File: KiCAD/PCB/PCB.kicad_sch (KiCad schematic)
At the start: 20 parts, among them J1 XLR3_AudioJack3_Combo_Switch, J2 Conn_01x04, J3 Conn_01x04, SW1 RotaryEncoder_Switch, U1 ESP32-WROOM-32D, U2 MPU-6050, U3 MIC5219-3.3YM5

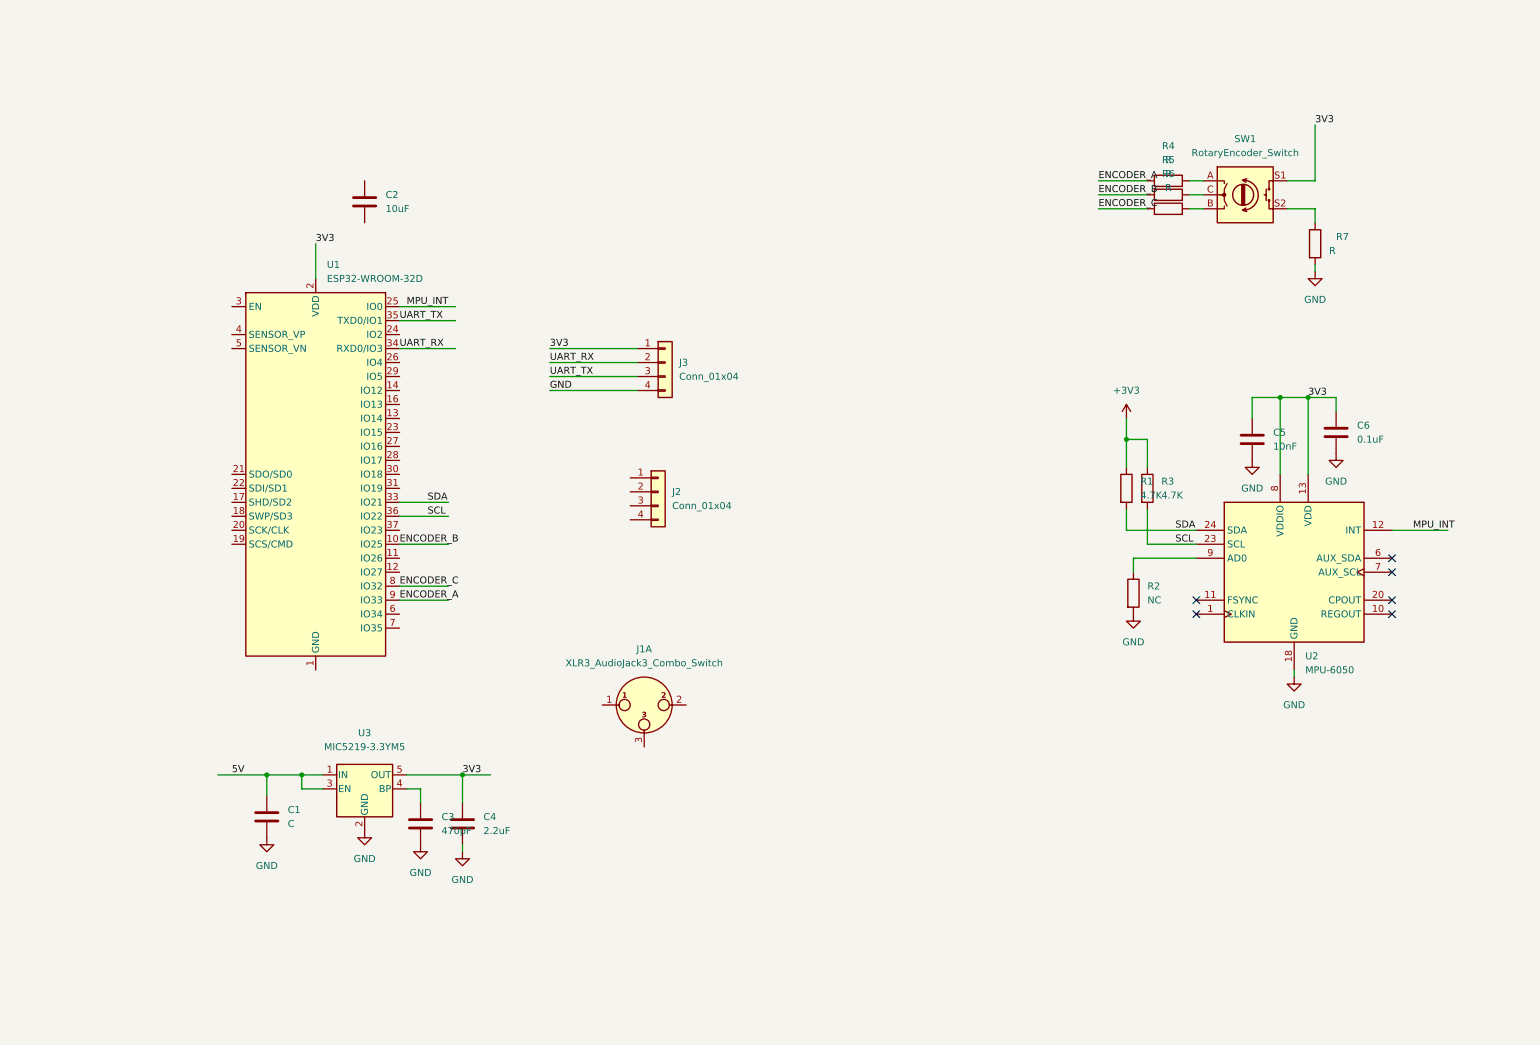
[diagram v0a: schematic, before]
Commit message: 原理圖第一版完成
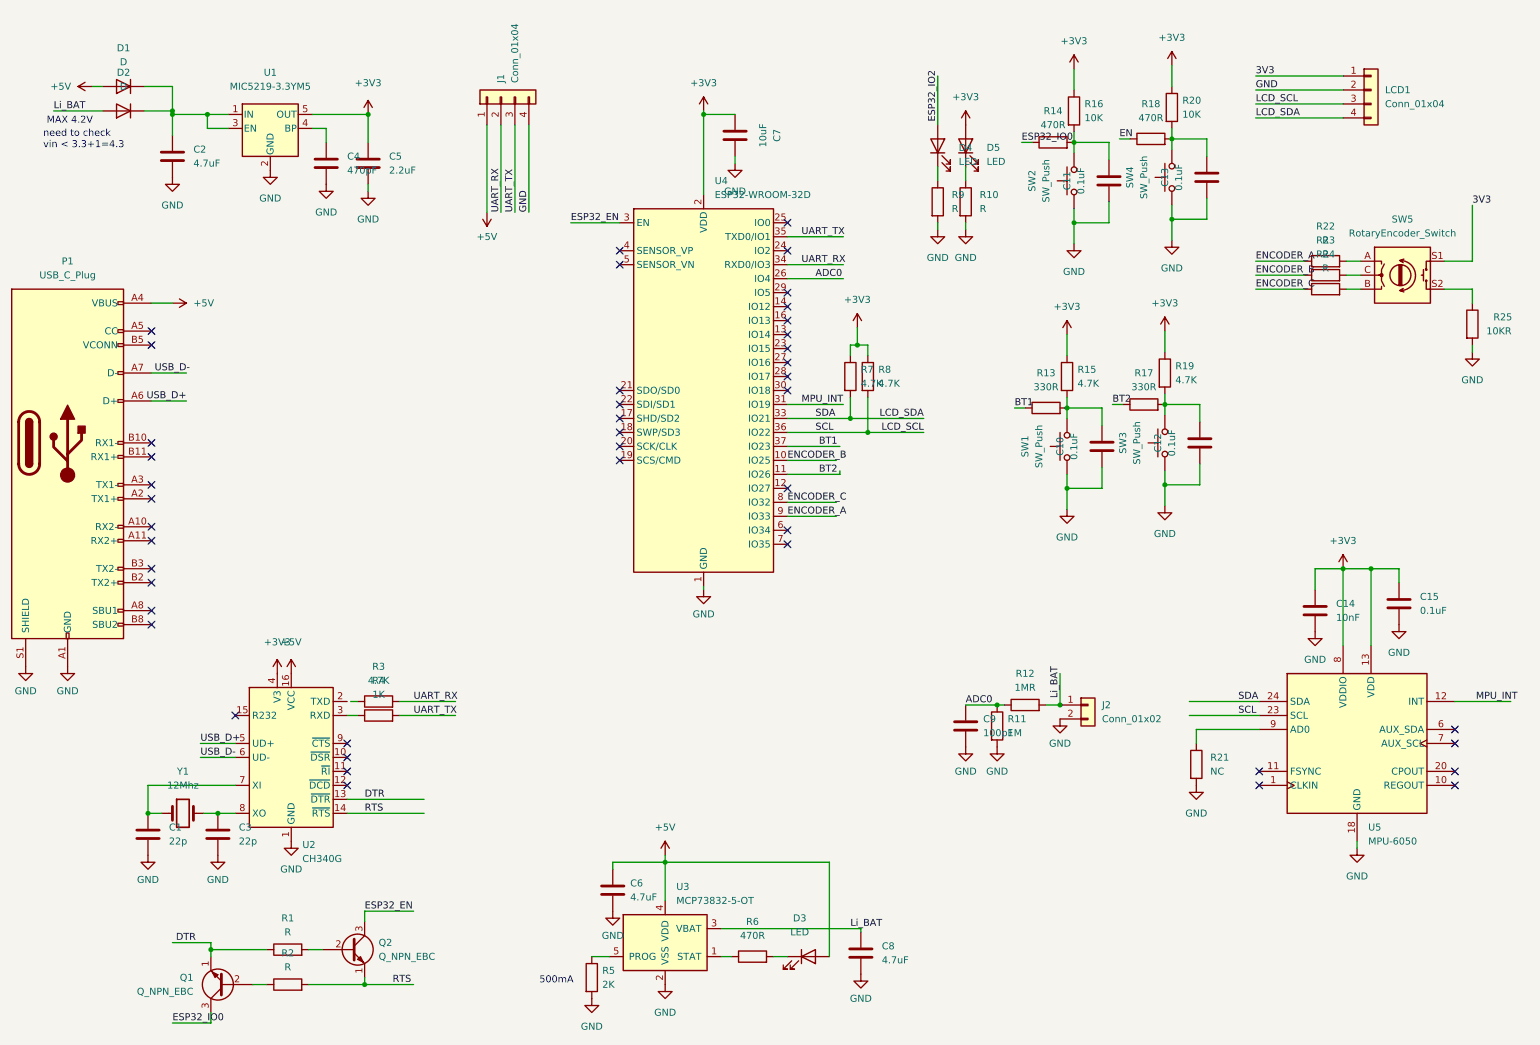
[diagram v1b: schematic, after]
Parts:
- removed J1: XLR3_AudioJack3_Combo_Switch, Button_Switch_THT:SW_E-Switch_EG2219_DPDT_Angled, symbol Connector:XLR3_AudioJack3_Combo_Switch
- added C1, C3: 22p, Capacitor_SMD:C_0603_1608Metric, symbol Device:C
- added C10, C11, C12, C13: 0.1uF, Capacitor_SMD:C_0603_1608Metric, symbol Device:C
- added C6, C8: 4.7uF, Capacitor_SMD:C_0603_1608Metric, symbol Device:C
- added C9: 100pF, Capacitor_SMD:C_0603_1608Metric, symbol Device:C
- added D1, D2: D, Diode_SMD:D_SMC_Handsoldering, symbol Device:D
- added D3, D4, D5: LED, LED_SMD:LED_0201_0603Metric, symbol Device:LED
- added J2: Conn_01x02, Connector_PinHeader_1.00mm:PinHeader_1x02_P1.00mm_Horizontal, symbol Connector_Generic:Conn_01x02
- added P1: USB_C_Plug, Connector_USB:HRI_TYPE_C, symbol Connector:USB_C_Plug
- added Q1, Q2: Q_NPN_EBC, Capacitor_SMD:C_0201_0603Metric, symbol Device:Q_NPN_EBC
- added R10, R2, R9: R, Capacitor_SMD:C_0201_0603Metric, symbol Device:R
- added R11: 1M, Capacitor_SMD:C_0201_0603Metric, symbol Device:R
- added R12: 1MR, Capacitor_SMD:C_0201_0603Metric, symbol Device:R
- added R13, R17: 330R, Capacitor_SMD:C_0201_0603Metric, symbol Device:R
- added R14, R18, R6: 470R, Capacitor_SMD:C_0201_0603Metric, symbol Device:R
- added R15, R19, R7, R8: 4.7K, Capacitor_SMD:C_0201_0603Metric, symbol Device:R
- added R16, R20: 10K, Capacitor_SMD:C_0201_0603Metric, symbol Device:R
- added R4: 1K, Capacitor_SMD:C_0201_0603Metric, symbol Device:R
- added R5: 2K, Capacitor_SMD:C_0201_0603Metric, symbol Device:R
- added SW1, SW2, SW3, SW4: SW_Push, Button_Switch_SMD:SW_Push_1P1T-SH_NO_CK_KMR2xxG, symbol Switch:SW_Push
- added U2: CH340G, Package_SO:SOIC-16_3.9x9.9mm_P1.27mm, symbol Interface_USB:CH340G
- added U3: MCP73832-5-OT, Package_TO_SOT_SMD:SOT-23-5, symbol Battery_Management:MCP73832-5-OT
- added Y1: 12Mhz, Crystal:Crystal_SMD_HC49-SD_HandSoldering, symbol Device:Crystal
- C2: renamed from C1; value C -> 4.7uF
- J1: renamed from J3; footprint (none) -> Connector_PinHeader_1.00mm:PinHeader_1x04_P1.00mm_Horizontal
- R1: value 4.7K -> R; footprint Resistor_SMD:R_0603_1608Metric -> Capacitor_SMD:C_0201_0603Metric
- R21: renamed from R2; footprint Resistor_SMD:R_0603_1608Metric -> Capacitor_SMD:C_0201_0603Metric
- R22: renamed from R4; footprint Resistor_SMD:R_0603_1608Metric -> Capacitor_SMD:C_0201_0603Metric
- R23: renamed from R5; footprint Resistor_SMD:R_0603_1608Metric -> Capacitor_SMD:C_0201_0603Metric
- R24: renamed from R6; footprint Resistor_SMD:R_0603_1608Metric -> Capacitor_SMD:C_0201_0603Metric
- R25: renamed from R7; value R -> 10KR; footprint Resistor_SMD:R_0603_1608Metric -> Capacitor_SMD:C_0201_0603Metric
- R3: footprint Resistor_SMD:R_0603_1608Metric -> Capacitor_SMD:C_0201_0603Metric
- renumbered C5 to C14, C6 to C15, C3 to C4, C4 to C5, C2 to C7, J2 to LCD1, SW1 to SW5, U3 to U1, U1 to U4, U2 to U5
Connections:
- net +3V3: now also C14.1, C15.1, C5.1, C7.1, U1.5 (OUT), U4.2 (VDD), U5.13 (VDD), U5.8 (VDDIO), D5.2 (A), R15.1, R16.1, R19.1, R20.1, R7.1, R8.1, U2.4 (V3); no longer R1.1, R3.1
- net 3V3: now also LCD1.1 (Pin_1); no longer C14.1, C15.1, C5.1, J1.1 (Pin_1), U1.5 (OUT), U4.2 (VDD), U5.13 (VDD), U5.8 (VDDIO)
- net GND: now also C7.2, LCD1.2 (Pin_2), U4.1 (GND), U4.15 (GND), U4.38 (GND), U4.39 (GND), C1.2, C10.1, C11.1, C12.1, C13.1, C3.2, C6.2, C8.2, C9.2, J2.2 (Pin_2), P1.A1 (GND), P1.A12 (GND), P1.B1 (GND), P1.B12 (GND), P1.S1 (SHIELD), R10.2, R11.2, R5.2, R9.2, SW1.1, SW2.1, SW3.1, SW4.1, U2.1 (GND), U3.2 (VSS)
- net MPU_INT: now also U4.31 (IO19); no longer U4.25 (IO0)
- net UART_RX: now also R3.2
- net UART_TX: now also R4.2
- net BT2: now reaches U4.11 (IO26)
- net BT2: now also R17.1
- net ADC0: now reaches U4.26 (IO4)
- net ADC0: now also C9.1, R11.1, R12.1
- net ESP32_EN: now reaches U4.3 (EN)
- net ESP32_EN: now also Q2.3 (C)
- net BT1: now reaches U4.37 (IO23)
- net BT1: now also R13.1
- net LCD_SCL: now reaches LCD1.3 (Pin_3)
- net LCD_SCL: now also U4.36 (IO22), U5.23 (SCL), R8.2
- net LCD_SDA: now reaches LCD1.4 (Pin_4)
- net LCD_SDA: now also U4.33 (IO21), U5.24 (SDA), R7.2
- net 5V: no longer names the net of C2.1, U1.1 (IN), U1.3 (EN)
- net 5V: now also D1.1 (K), D2.1 (K)
- removed net SCL: R3.2, U4.36 (IO22), U5.23 (SCL)
- removed net SDA: R1.2, U4.33 (IO21), U5.24 (SDA)
- new net: C12.2, R17.2, R19.2, SW3.2
- new net: D5.1 (K), R10.1
- new net: C1.1, U2.7 (XI), Y1.1
- new net: C3.1, U2.8 (XO), Y1.2
- new net: C10.2, R13.2, R15.2, SW1.2
- new net: D4.1 (K), R9.1
- new net: C11.2, R14.2, R16.2, SW2.2
- new net: R4.1, U2.3 (RXD)
- new net: C13.2, R18.2, R20.2, SW4.2
- new net: Q2.2 (B), R1.2
- new net: D3.1 (K), R6.2
- new net: Q1.2 (B), R2.1
- new net: R6.1, U3.1 (STAT)
- new net: R5.1, U3.5 (PROG)
- new net +5V: C6.1, D1.2 (A), D3.2 (A), J1.1 (Pin_1), P1.A4 (VBUS), P1.A9 (VBUS), P1.B4 (VBUS), P1.B9 (VBUS), U2.16 (VCC), U3.4 (VDD)
- new net DTR: Q1.1 (E), R1.1, U2.13 (~{DTR})
- new net EN: R18.1
- new net ESP32_IO0: Q1.3 (C), R14.1
- new net ESP32_IO2: D4.2 (A)
- new net Li_BAT: C8.1, D2.2 (A), J2.1 (Pin_1), R12.2, U3.3 (VBAT)
- new net RTS: Q2.1 (E), R2.2, U2.14 (~{RTS})
- new net USB_D+: P1.A6 (D+), U2.5 (UD+)
- new net USB_D-: U2.6 (UD-)
- no-connect marks 6 -> 44
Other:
- note added: "500mA"
- note added: "MAX 4.2V"
- note added: "need to check vin < 3.3+1=4.3"
- moved on the sheet: C14, C15, C2, C4, C5, C7, J1, LCD1, R21, R22, R23, R24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
